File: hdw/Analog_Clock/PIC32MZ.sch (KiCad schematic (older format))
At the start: 1 part

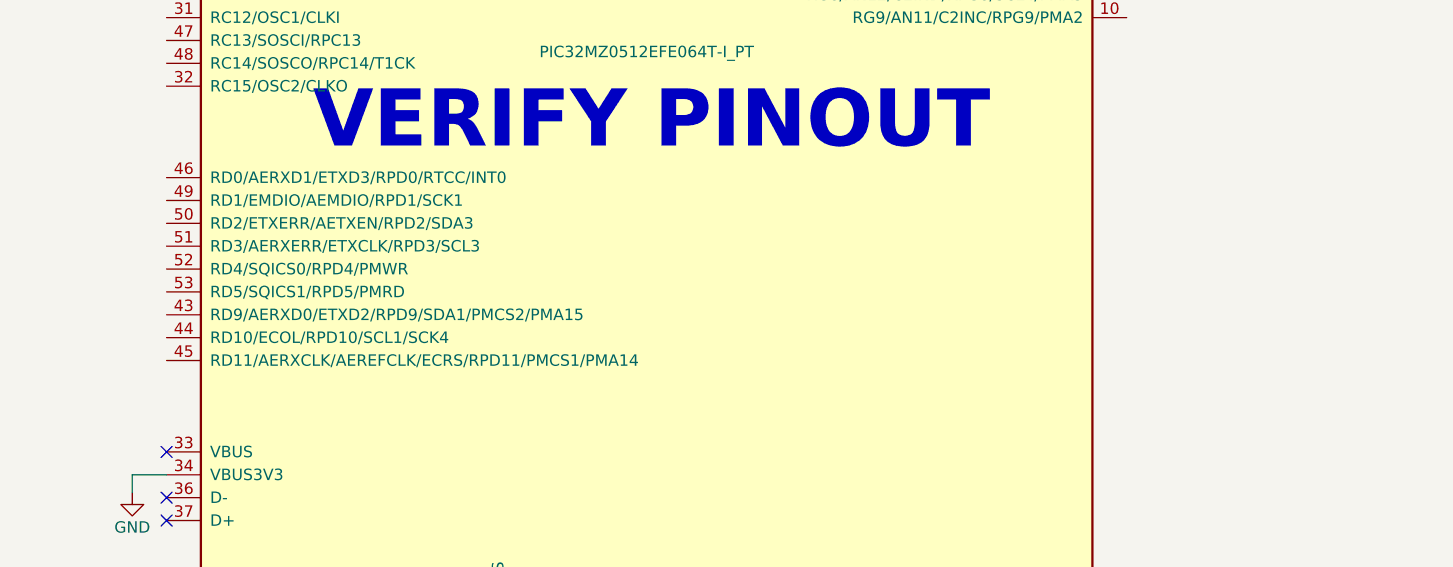
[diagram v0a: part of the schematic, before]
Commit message: More schematic work
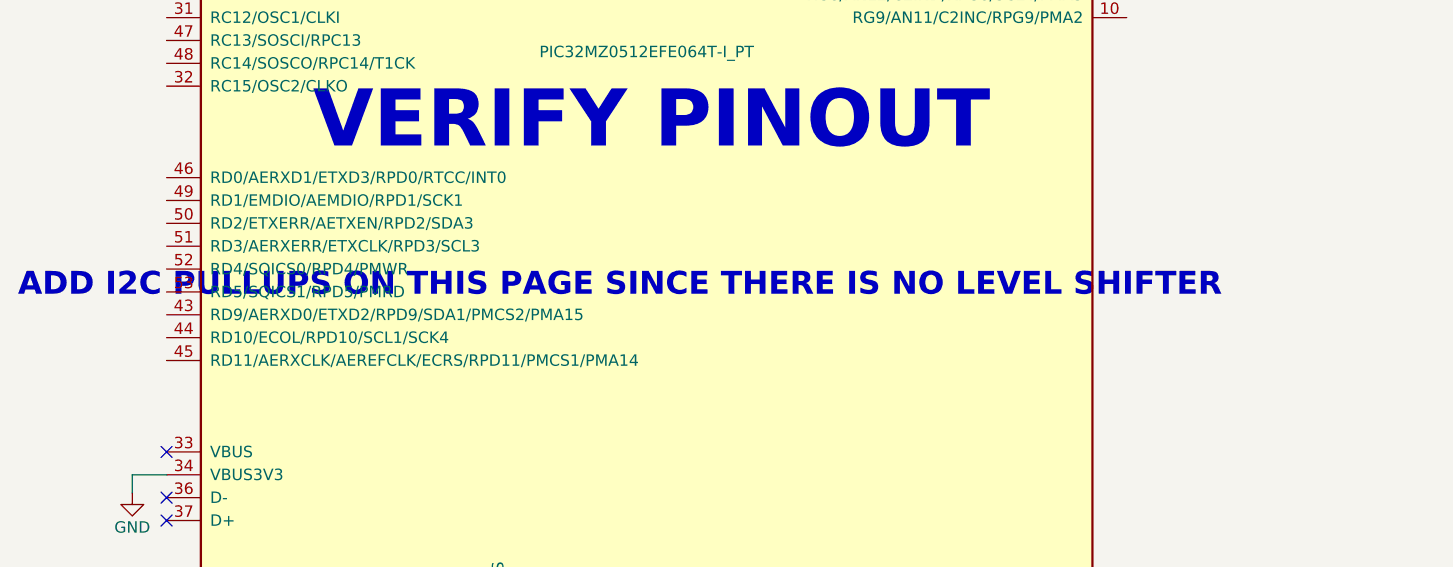
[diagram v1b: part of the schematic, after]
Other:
- note added: "ADD I2C PULLUPS ON THIS PAGE SINCE THERE IS NO LEVEL SHIFTER"
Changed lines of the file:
@@
 EESchema Schematic File Version 4
+LIBS:Analog_Clock-cache
 EELAYER 30 0
 EELAYER END
@@
 	1    0    0    -1
 $EndComp
+Text Notes 2710 4640 0    100  ~ 20
+ADD I2C PULLUPS ON THIS PAGE SINCE THERE IS NO LEVEL SHIFTER
 $EndSCHEMATC

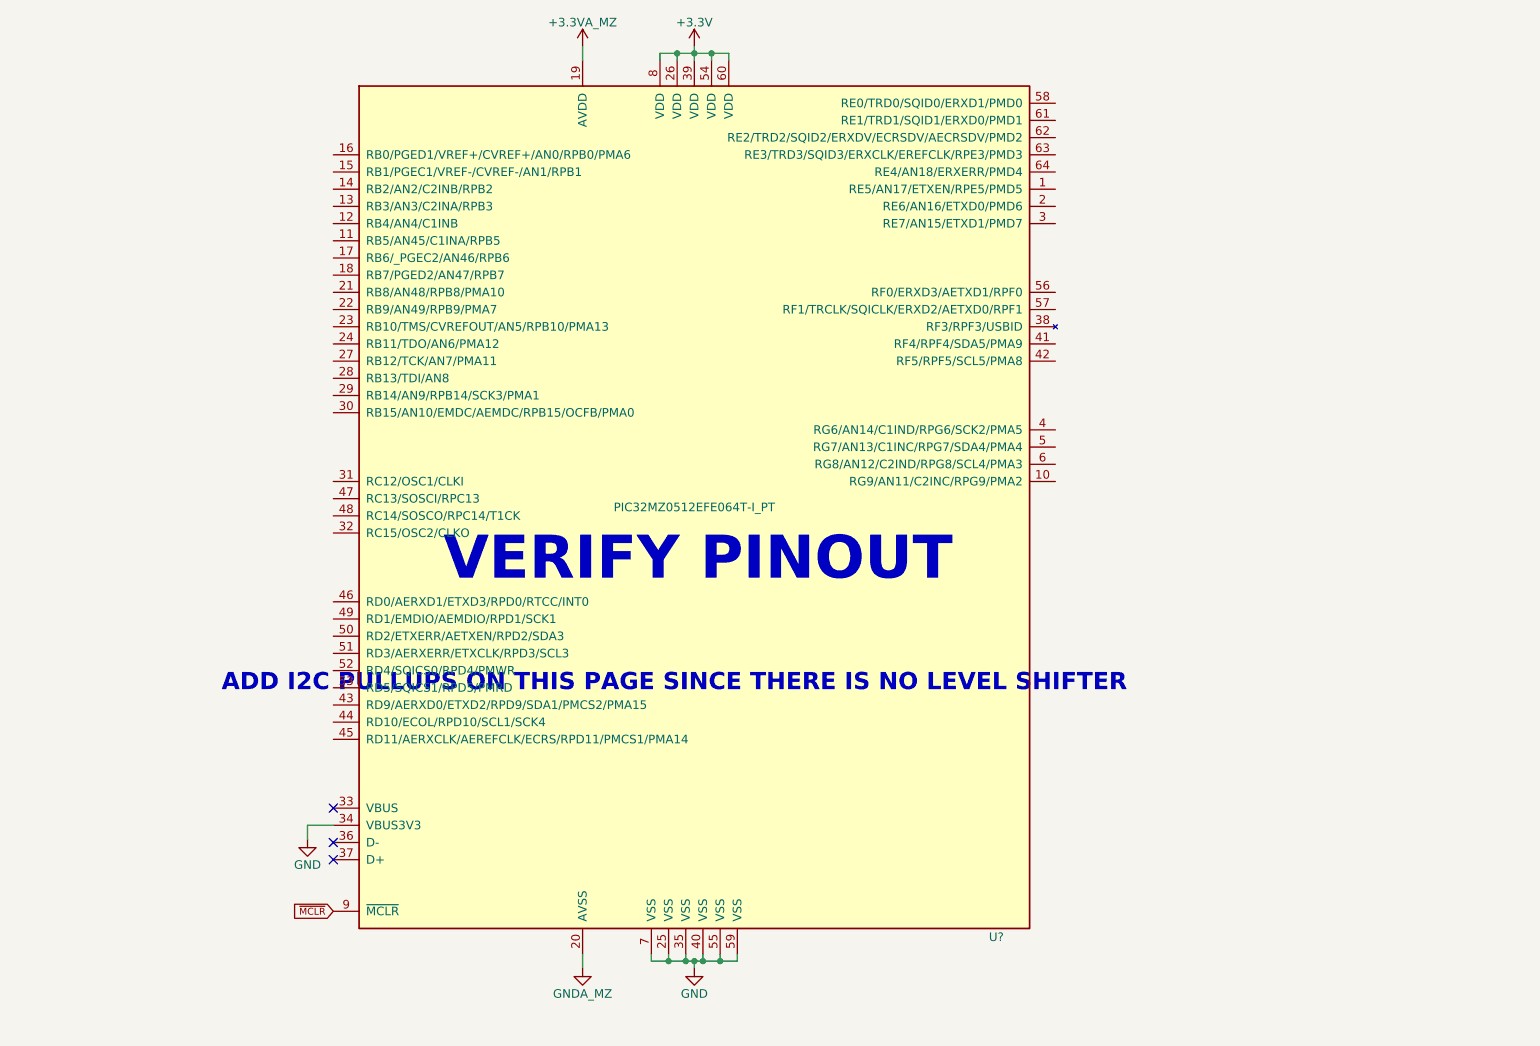
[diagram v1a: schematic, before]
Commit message: a few sch adjustments
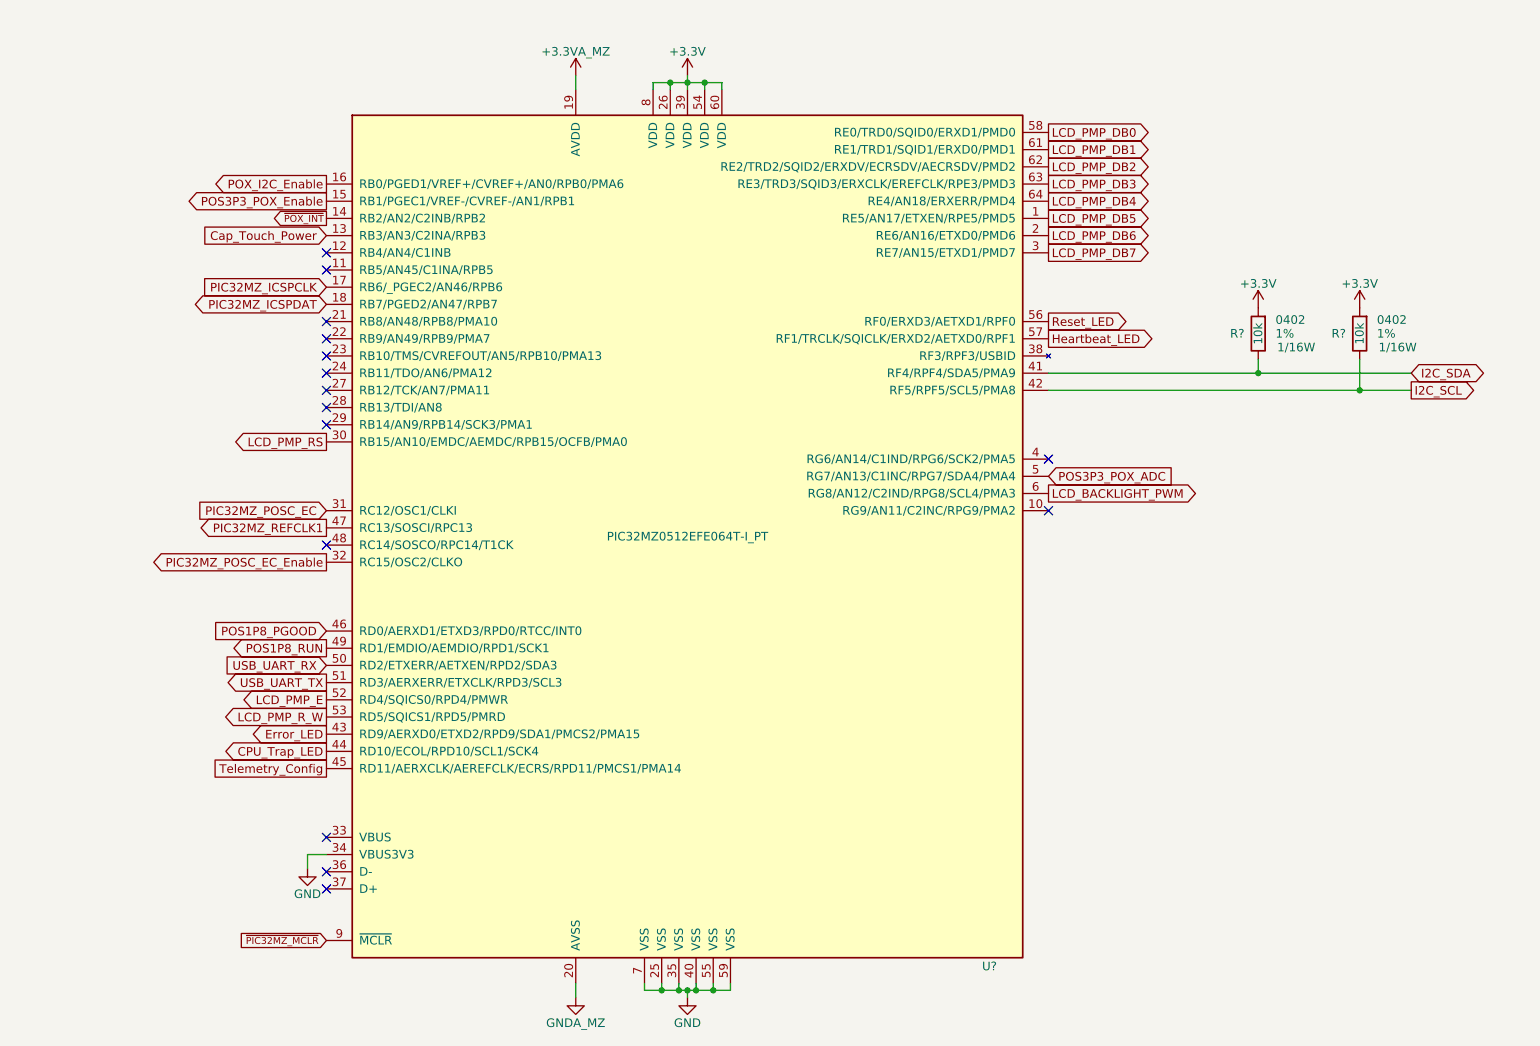
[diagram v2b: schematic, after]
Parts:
- removed U?: PIC32MZ0512EFE064T-I_PT, Package_QFP:TQFP-64_10x10mm_P0.5mm, symbol Custom_Library:PIC32MZ0512EFE064T-I_PT
- added R? (x2): 10k, Resistors_SMD:R_0402, symbol Custom_Library:R_Custom
- added U?: PIC32MZ0512EFE064T-I_PT, Package_QFP:TQFP-64_10x10mm_P0.5mm, symbol Custom_Library:PIC32MZ0512EFE064T-I_PT
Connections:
- net +3.3VA_MZ: now also U?.19 (AVDD)
- net +3V3: now also R?.1, R?.1, U?.26 (VDD), U?.39 (VDD), U?.54 (VDD), U?.60 (VDD), U?.8 (VDD)
- net GND: now also U?.25 (VSS), U?.34 (VBUS3V3), U?.35 (VSS), U?.40 (VSS), U?.55 (VSS), U?.59 (VSS), U?.7 (VSS)
- net GNDA_MZ: now also U?.20 (AVSS)
- new net CPU_Trap_LED: U?.44 (RD10/ECOL/RPD10/SCL1/SCK4)
- new net Cap_Touch_Power: U?.13 (RB3/AN3/C2INA/RPB3)
- new net Error_LED: U?.43 (RD9/AERXD0/ETXD2/RPD9/SDA1/PMCS2/PMA15)
- new net Heartbeat_LED: U?.57 (RF1/TRCLK/SQICLK/ERXD2/AETXD0/RPF1)
- new net I2C_SCL: R?.2, U?.42 (RF5/RPF5/SCL5/PMA8)
- new net I2C_SDA: R?.2, U?.41 (RF4/RPF4/SDA5/PMA9)
- new net LCD_BACKLIGHT_PWM: U?.6 (RG8/AN12/C2IND/RPG8/SCL4/PMA3)
- new net LCD_PMP_DB0: U?.58 (RE0/TRD0/SQID0/ERXD1/PMD0)
- new net LCD_PMP_DB1: U?.61 (RE1/TRD1/SQID1/ERXD0/PMD1)
- new net LCD_PMP_DB2: U?.62 (RE2/TRD2/SQID2/ERXDV/ECRSDV/AECRSDV/PMD2)
- new net LCD_PMP_DB3: U?.63 (RE3/TRD3/SQID3/ERXCLK/EREFCLK/RPE3/PMD3)
- new net LCD_PMP_DB4: U?.64 (RE4/AN18/ERXERR/PMD4)
- new net LCD_PMP_DB5: U?.1 (RE5/AN17/ETXEN/RPE5/PMD5)
- new net LCD_PMP_DB6: U?.2 (RE6/AN16/ETXD0/PMD6)
- new net LCD_PMP_DB7: U?.3 (RE7/AN15/ETXD1/PMD7)
- new net LCD_PMP_E: U?.52 (RD4/SQICS0/RPD4/PMWR)
- new net LCD_PMP_RS: U?.30 (RB15/AN10/EMDC/AEMDC/RPB15/OCFB/PMA0)
- new net LCD_PMP_R_W: U?.53 (RD5/SQICS1/RPD5/PMRD)
- new net PIC32MZ_ICSPCLK: U?.17 (RB6/_PGEC2/AN46/RPB6)
- new net PIC32MZ_ICSPDAT: U?.18 (RB7/PGED2/AN47/RPB7)
- new net PIC32MZ_POSC_EC: U?.31 (RC12/OSC1/CLKI)
- new net PIC32MZ_POSC_EC_Enable: U?.32 (RC15/OSC2/CLKO)
- new net PIC32MZ_REFCLK1: U?.47 (RC13/SOSCI/RPC13)
- new net POS1P8_PGOOD: U?.46 (RD0/AERXD1/ETXD3/RPD0/RTCC/INT0)
- new net POS1P8_RUN: U?.49 (RD1/EMDIO/AEMDIO/RPD1/SCK1)
- new net POS3P3_POX_ADC: U?.5 (RG7/AN13/C1INC/RPG7/SDA4/PMA4)
- new net POS3P3_POX_Enable: U?.15 (RB1/PGEC1/VREF-/CVREF-/AN1/RPB1)
- new net POX_I2C_Enable: U?.16 (RB0/PGED1/VREF+/CVREF+/AN0/RPB0/PMA6)
- new net Reset_LED: U?.56 (RF0/ERXD3/AETXD1/RPF0)
- new net Telemetry_Config: U?.45 (RD11/AERXCLK/AEREFCLK/ECRS/RPD11/PMCS1/PMA14)
- new net USB_UART_RX: U?.50 (RD2/ETXERR/AETXEN/RPD2/SDA3)
- new net USB_UART_TX: U?.51 (RD3/AERXERR/ETXCLK/RPD3/SCL3)
- new net ~PIC32MZ_MCLR: U?.9 (~MCLR~)
- new net ~POX_INT: U?.14 (RB2/AN2/C2INB/RPB2)
- no-connect marks 3 -> 15
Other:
- note removed: "ADD I2C PULLUPS ON THIS PAGE SINCE THERE IS NO LEVEL SHIFTER"
- note removed: "VERIFY PINOUT"

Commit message: More sch work
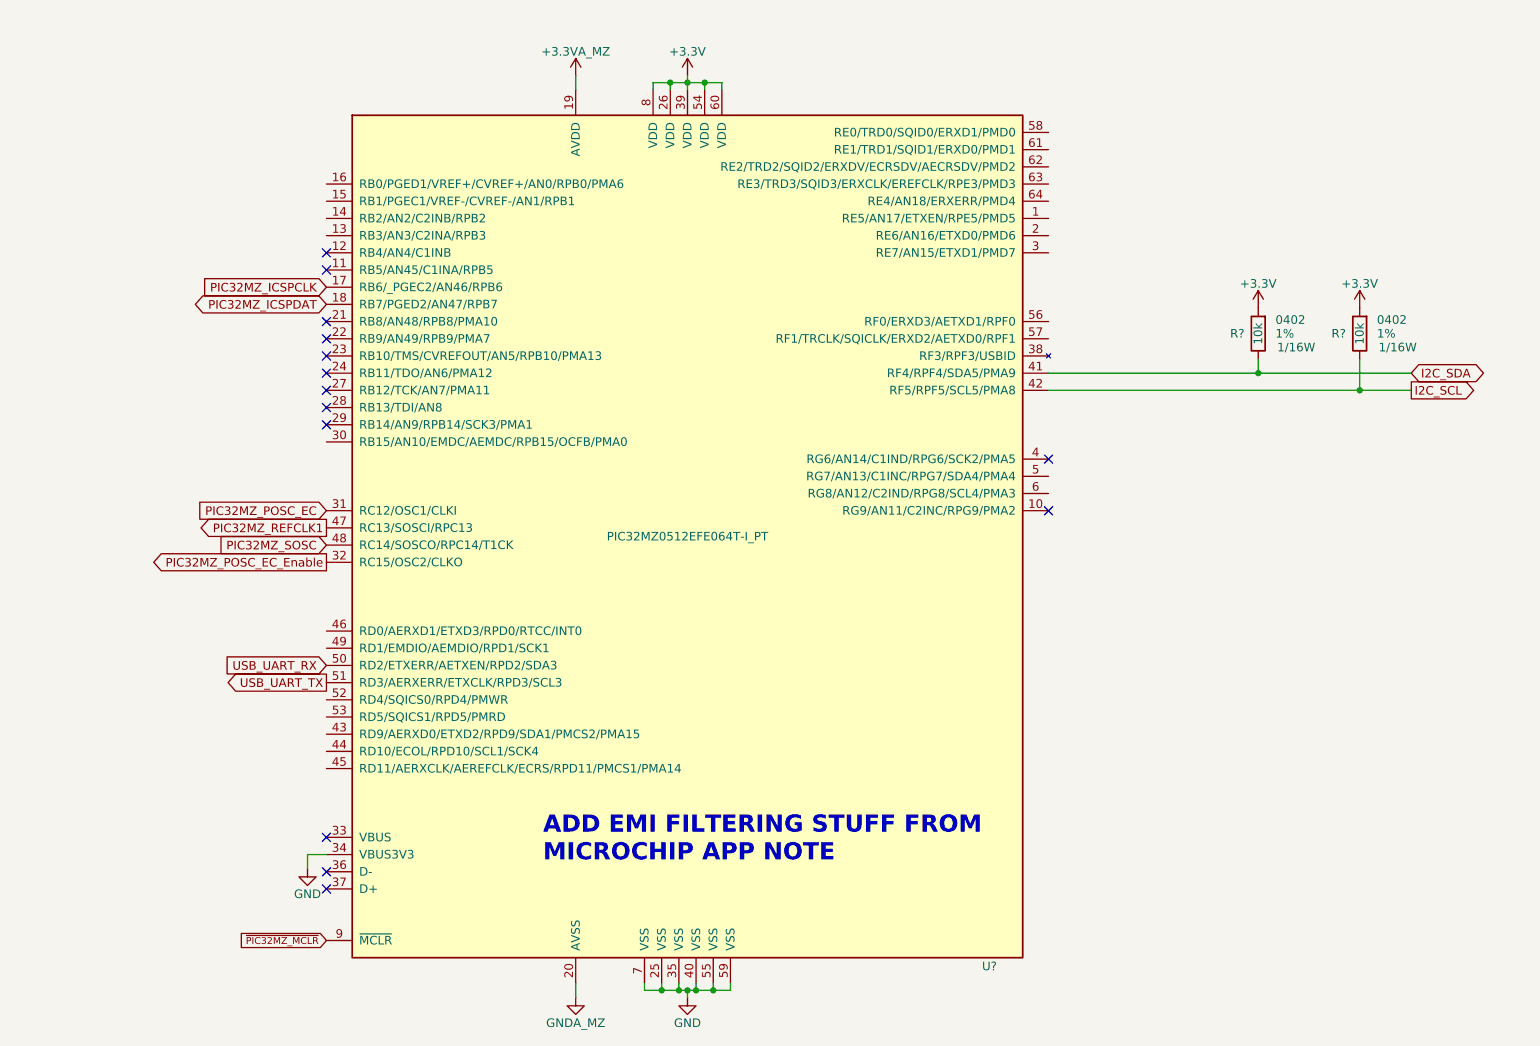
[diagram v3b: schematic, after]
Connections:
- net PIC32MZ_SOSC: now reaches U?.48 (RC14/SOSCO/RPC14/T1CK)
- net CPU_Trap_LED: no longer names the net of U?.44 (RD10/ECOL/RPD10/SCL1/SCK4)
- net Cap_Touch_Power: no longer names the net of U?.13 (RB3/AN3/C2INA/RPB3)
- net Error_LED: no longer names the net of U?.43 (RD9/AERXD0/ETXD2/RPD9/SDA1/PMCS2/PMA15)
- net Heartbeat_LED: no longer names the net of U?.57 (RF1/TRCLK/SQICLK/ERXD2/AETXD0/RPF1)
- net LCD_BACKLIGHT_PWM: no longer names the net of U?.6 (RG8/AN12/C2IND/RPG8/SCL4/PMA3)
- net LCD_PMP_DB0: no longer names the net of U?.58 (RE0/TRD0/SQID0/ERXD1/PMD0)
- net LCD_PMP_DB1: no longer names the net of U?.61 (RE1/TRD1/SQID1/ERXD0/PMD1)
- net LCD_PMP_DB2: no longer names the net of U?.62 (RE2/TRD2/SQID2/ERXDV/ECRSDV/AECRSDV/PMD2)
- net LCD_PMP_DB3: no longer names the net of U?.63 (RE3/TRD3/SQID3/ERXCLK/EREFCLK/RPE3/PMD3)
- net LCD_PMP_DB4: no longer names the net of U?.64 (RE4/AN18/ERXERR/PMD4)
- net LCD_PMP_DB5: no longer names the net of U?.1 (RE5/AN17/ETXEN/RPE5/PMD5)
- net LCD_PMP_DB6: no longer names the net of U?.2 (RE6/AN16/ETXD0/PMD6)
- net LCD_PMP_DB7: no longer names the net of U?.3 (RE7/AN15/ETXD1/PMD7)
- net LCD_PMP_E: no longer names the net of U?.52 (RD4/SQICS0/RPD4/PMWR)
- net LCD_PMP_RS: no longer names the net of U?.30 (RB15/AN10/EMDC/AEMDC/RPB15/OCFB/PMA0)
- net LCD_PMP_R_W: no longer names the net of U?.53 (RD5/SQICS1/RPD5/PMRD)
- net POS1P8_PGOOD: no longer names the net of U?.46 (RD0/AERXD1/ETXD3/RPD0/RTCC/INT0)
- net POS1P8_RUN: no longer names the net of U?.49 (RD1/EMDIO/AEMDIO/RPD1/SCK1)
- net POS3P3_POX_ADC: no longer names the net of U?.5 (RG7/AN13/C1INC/RPG7/SDA4/PMA4)
- net POS3P3_POX_Enable: no longer names the net of U?.15 (RB1/PGEC1/VREF-/CVREF-/AN1/RPB1)
- net POX_I2C_Enable: no longer names the net of U?.16 (RB0/PGED1/VREF+/CVREF+/AN0/RPB0/PMA6)
- net Reset_LED: no longer names the net of U?.56 (RF0/ERXD3/AETXD1/RPF0)
- net Telemetry_Config: no longer names the net of U?.45 (RD11/AERXCLK/AEREFCLK/ECRS/RPD11/PMCS1/PMA14)
- net ~POX_INT: no longer names the net of U?.14 (RB2/AN2/C2INB/RPB2)
- no-connect marks 15 -> 14
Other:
- note added: "ADD EMI FILTERING STUFF FROM\nMICROCHIP APP NOTE"
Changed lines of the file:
@@
 $Descr A 11000 8500
 encoding utf-8
-Sheet 11 20
+Sheet 10 21
 Title "Pulse Oximeter"
 Date "2020-08-01"
@@
 	1    0    0    -1
 $EndComp
-Text GLabel 7520 3480 2    50   Output ~ 0
-LCD_BACKLIGHT_PWM
-Text GLabel 3320 3180 0    50   Output ~ 0
-LCD_PMP_RS
-Text GLabel 3320 4780 0    50   Output ~ 0
-LCD_PMP_R_W
-Text GLabel 3320 4680 0    50   Output ~ 0
-LCD_PMP_E
-Text GLabel 7520 1380 2    50   Output ~ 0
-LCD_PMP_DB0
-Text GLabel 7520 1480 2    50   Output ~ 0
-LCD_PMP_DB1
-Text GLabel 7520 1580 2    50   Output ~ 0
-LCD_PMP_DB2
-Text GLabel 7520 1680 2    50   Output ~ 0
-LCD_PMP_DB3
-Text GLabel 7520 1780 2    50   Output ~ 0
-LCD_PMP_DB4
-Text GLabel 7520 1880 2    50   Output ~ 0
-LCD_PMP_DB5
-Text GLabel 7520 1980 2    50   Output ~ 0
-LCD_PMP_DB6
-Text GLabel 7520 2080 2    50   Output ~ 0
-LCD_PMP_DB7
 Text GLabel 3320 3680 0    50   Output ~ 0
 PIC32MZ_REFCLK1
@@
 AR Path="/5EAE4A89/5EB7DAD1" Ref="R?"  Part="1"
 AR Path="/5EAE2F23/5EB7DAD1" Ref="R?"  Part="1"
+AR Path="/5E939ED2/5EB7DAD1" Ref="R?"  Part="1"
 F 0 "R?" H 9250 2550 50  0000 R CNN
 F 1 "10k" V 9330 2550 50  0000 C CNN
@@
 AR Path="/5EAE4A89/5EB7DEAB" Ref="R?"  Part="1"
 AR Path="/5EAE2F23/5EB7DEAB" Ref="R?"  Part="1"
+AR Path="/5E939ED2/5EB7DEAB" Ref="R?"  Part="1"
 F 0 "R?" H 8660 2550 50  0000 R CNN
 F 1 "10k" V 8740 2550 50  0000 C CNN
@@
 Wire Wire Line
 	9330 2880 9630 2880
-Text GLabel 3320 5080 0    50   UnSpc ~ 0
-Telemetry_Config
-Text GLabel 3320 4280 0    50   Input ~ 0
-POS1P8_PGOOD
-Text GLabel 3320 4380 0    50   Output ~ 0
-POS1P8_RUN
-Text GLabel 3320 1680 0    50   Output ~ 0
-POX_I2C_Enable
-Text GLabel 3320 1780 0    50   Output ~ 0
-POS3P3_POX_Enable
-Text GLabel 3320 1880 0    40   Output ~ 0
-~POX_INT
-Text GLabel 3320 1980 0    50   Input ~ 0
-Cap_Touch_Power
-Text GLabel 7520 2480 2    50   Output ~ 0
-Reset_LED
-Text GLabel 3320 4980 0    50   Output ~ 0
-CPU_Trap_LED
-Text GLabel 7520 2580 2    50   Output ~ 0
-Heartbeat_LED
-Text GLabel 3320 4880 0    50   Output ~ 0
-Error_LED
-Text GLabel 7520 3380 2    50   Input ~ 0
-POS3P3_POX_ADC
 NoConn ~ 3320 2080
 NoConn ~ 3320 2180
 NoConn ~ 3320 2780
 NoConn ~ 3320 2880
-NoConn ~ 3320 3780
 NoConn ~ 7520 3280
 NoConn ~ 7520 3580
@@
 NoConn ~ 3320 2980
 NoConn ~ 3320 3080
+Text Notes 4580 5630 0    100  ~ 20
+ADD EMI FILTERING STUFF FROM\nMICROCHIP APP NOTE
+Text GLabel 3320 3780 0    50   Input ~ 0
+PIC32MZ_SOSC
 $EndSCHEMATC
